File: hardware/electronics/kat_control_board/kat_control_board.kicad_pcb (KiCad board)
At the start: 4 copper layers, 85 x 175 mm, 113 parts, among them J1 USB_C_Receptacle_USB2.0, J10 Conn_01x04, J11 Conn_01x04, J12 Conn_01x04, J13 Conn_01x04, J14 Conn_01x04, J15 Conn_01x04, J16 Conn_01x04, J17 Conn_01x02, J18 Conn_01x04, J19 Conn_01x04, J2 Conn_01x04, J20 Conn_01x02, J21 Conn_01x02, J22 Conn_01x02, J23 Conn_01x02, J24 Conn_01x02, J25 Conn_01x02, J26 Conn_01x02, J27 Conn_01x02, J3 Conn_01x04, J4 Conn_01x04, J5 Conn_01x04, J6 Conn_01x04, J7 Conn_01x04, J8 Conn_01x04, J9 Conn_01x04, Q1 AO3400A, Q2 AO3400A, Q3 AO3400A, Q4 AO3400A, Q5 AO3400A, SW1 SW_SPST, SW2 SW_SPST, U1 RP2040, U2 W25Q128JVS, U3 SN74HC4851, U4 74HCT244, U5 74HCT244, U6 SIC431, U7 XC6206PxxxMR, Y1 12MHz

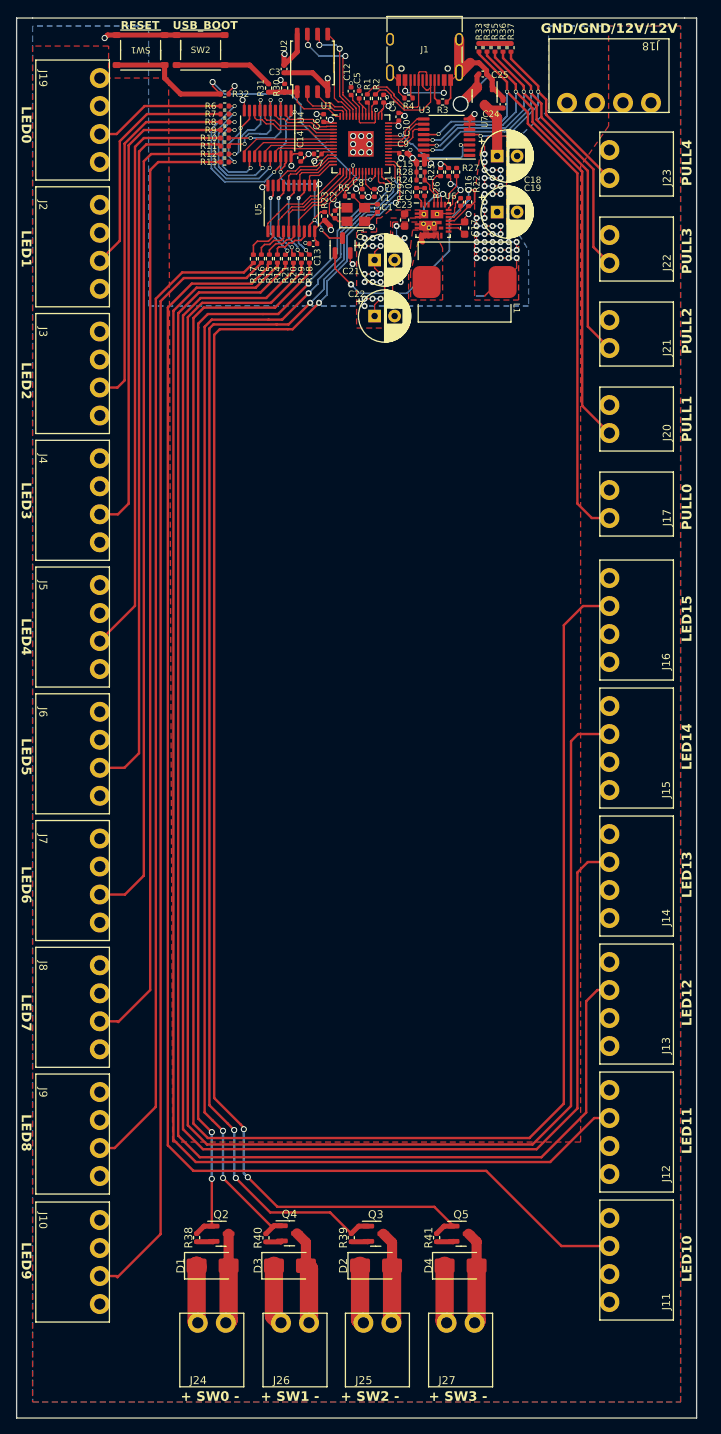
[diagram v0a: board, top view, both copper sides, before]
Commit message: Added rev1 PCB design
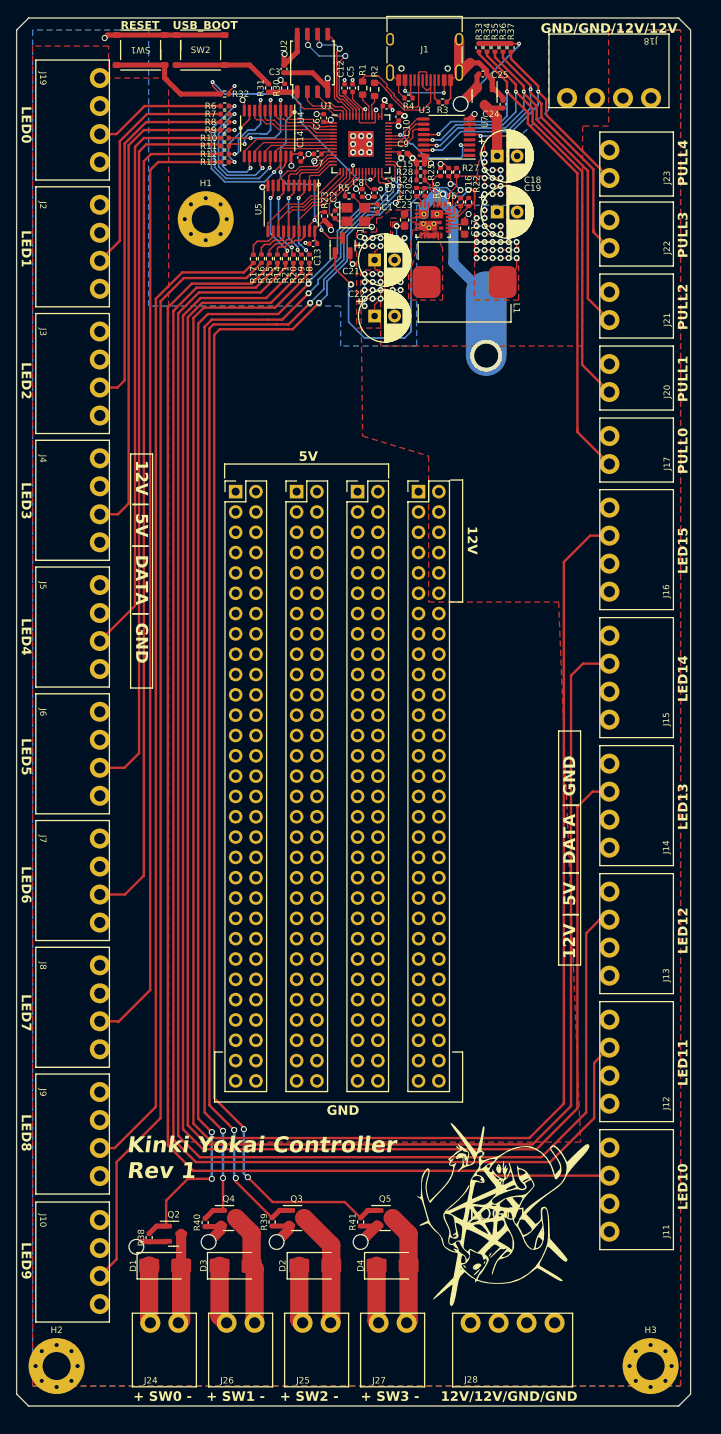
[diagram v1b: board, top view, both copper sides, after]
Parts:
- added H1: MountingHole, MountingHole:MountingHole_3.5mm_Pad_Via, F.Cu at (52.1, 42.1)
- added H2: MountingHole, MountingHole:MountingHole_3.5mm_Pad_Via, F.Cu at (33.5, 185.5)
- added H3: MountingHole, MountingHole:MountingHole_3.5mm_Pad_Via, F.Cu at (107.8, 185.5)
- added J28: Conn_01x04, M_Connectors:DB2ERC-3.5-4P, F.Cu at (90.5, 180.1)
- added J29: Conn_02x30_Odd_Even, Connector_PinHeader_2.54mm:PinHeader_2x30_P2.54mm_Vertical, F.Cu at (55.9, 76.2)
- added J30: Conn_02x30_Odd_Even, Connector_PinHeader_2.54mm:PinHeader_2x30_P2.54mm_Vertical, F.Cu at (63.5, 76.2)
- added J31: Conn_02x30_Odd_Even, Connector_PinHeader_2.54mm:PinHeader_2x30_P2.54mm_Vertical, F.Cu at (71.1, 76.2)
- added J32: Conn_02x30_Odd_Even, Connector_PinHeader_2.54mm:PinHeader_2x30_P2.54mm_Vertical, F.Cu at (78.7, 76.2)
- added LOGO1: Logo_Open_Hardware_Small, M_LOGOS:kinki_yokai_logo, F.Cu at (88.8, 166.5)
- R1, R2: value 27R4 -> 27R; footprint Resistor_SMD:R_0402_1005Metric -> Resistor_SMD:R_0603_1608Metric
- moved Q3 10.1 mm to (63.5, 167.0)
- moved R39 10.1 mm to (60.4, 167.5)
- moved Q5 9.70 mm to (74.6, 167.0)
- moved R41 9.70 mm to (71.5, 167.5)
- moved J11 8.80 mm to (102.6, 163.4)
- moved J12 8.80 mm to (102.6, 147.4)
- moved J13 8.80 mm to (102.6, 131.4)
- moved J14 8.80 mm to (102.6, 115.5)
- moved J15 8.80 mm to (102.6, 99.5)
- moved J16 8.80 mm to (102.6, 83.5)
- moved D4 8.50 mm to (75.5, 173.0)
- moved J27 8.50 mm to (75.5, 180.1)
- moved Q4 7.84 mm to (55.0, 167.0)
- moved R40 7.84 mm to (52.1, 167.6)
- moved D2 7.60 mm to (65.8, 173.0)
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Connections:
- net Net-(U1-GPIO23) renamed /AMUX_A
- net Net-(U1-GPIO24) renamed /AMUX_B
- net Net-(U1-GPIO25) renamed /AMUX_C
- net Net-(U1-GPIO26_ADC0) renamed /AMUX_X
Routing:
- net +12V: track 54.4 -> 83.3 mm, vias 17 -> 21
- net Net-(Q1-G): track 34.7 -> 49.7 mm
- net /SW3: track 176.6 -> 164.6 mm
- net /SW2: track 165.1 -> 154.6 mm
- net GND: track 114.3 -> 124.7 mm, vias 42 -> 47
- net /LED12: track 191.0 -> 199.6 mm
- net /LED14: track 220.4 -> 228.8 mm
- net /LED13: track 205.3 -> 213.8 mm
- net /LED15: track 234.2 -> 242.4 mm
- net /PULL0: track 80.9 -> 72.9 mm
- net /LED11: track 177.3 -> 185.0 mm
- net +3V3: track 44.8 -> 50.9 mm, vias 11 -> 13
- net /SW1: track 155.6 -> 149.9 mm
- net /PULL1: track 69.5 -> 64.4 mm
- net /SW0: track 151.6 -> 155.6 mm
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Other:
- board size 85 x 175 mm -> 84.2 x 173.5 mm
- board text added: "12V"
- board text added: "12V | 5V | DATA | GND"
- board text added: "12V/12V/GND/GND"
- board text added: "5V"
- board text added: "GND"
- board text added: "Kinki Yokai Controller Rev 1"
